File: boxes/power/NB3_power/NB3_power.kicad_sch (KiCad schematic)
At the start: 82 parts, among them J1 Barrel_Jack_PJ-036AH-SMT-TR, J2 Conn_01x02_Male, J3 Conn_01x02_Male, J4 Conn_01x02_Male, J5 Conn_01x04_Male, J6 Conn_01x02_Male, J7 Conn_01x02_Male, Q1 Q_PMOS_GDS, Q2 Q_NMOS_GDS, SW1 SW_SPDT, U1 NiMH_Charger_LTC4010, U2 Voltage_Regulator_AP64501

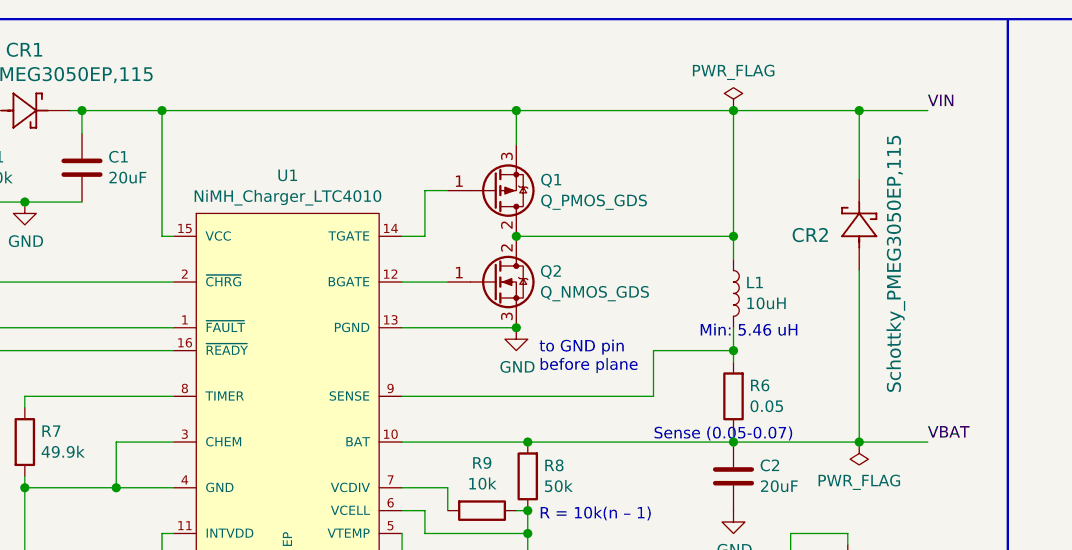
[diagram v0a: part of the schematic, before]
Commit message: More work on NB£_power PCB
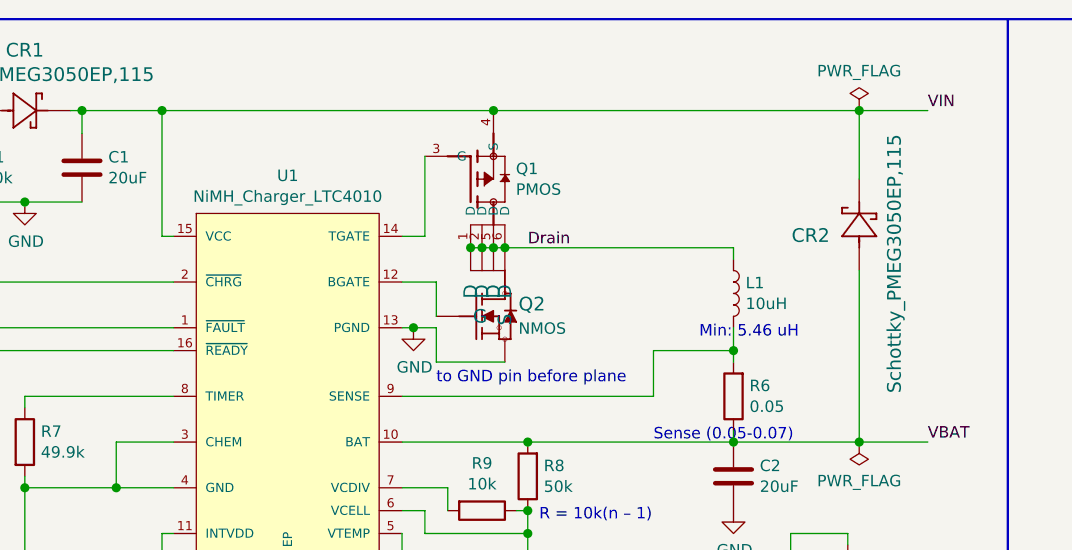
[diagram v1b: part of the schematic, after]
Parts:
- removed Q1: Q_PMOS_GDS, NB3_power:PMOS_SMD_FDC658AP, symbol Device:Q_PMOS_GDS
- removed Q2: Q_NMOS_GDS, NB3_power:NMOS_SMD_SI3410DV-T1-GE3, symbol Device:Q_NMOS_GDS
- added Q1: PMOS, NB3_power:PMOS_SMD_FDC658AP, symbol NB3_power:PMOS_SMD_FDC658AP
- added Q2: NMOS, NB3_power:NMOS_SMD_SI3410DV-T1-GE3, symbol NB3_power:NMOS_SMD_SI3410DV-T1-GE3
- J2, J3, J4, J6, J7: footprint Connector_PinHeader_2.54mm:PinHeader_1x02_P2.54mm_Vertical_SMD_Pin1Left -> Connector_PinHeader_2.54mm:PinHeader_1x02_P2.54mm_Vertical_SMD_Pin1Right
- J5: footprint Connector_PinHeader_2.54mm:PinHeader_1x04_P2.54mm_Vertical_SMD_Pin1Left -> Connector_PinHeader_2.54mm:PinHeader_1x04_P2.54mm_Vertical_SMD_Pin1Right
- L1: footprint Inductor_SMD:L_0805_2012Metric -> Inductor_SMD:L_Bourns_SRN6045TA
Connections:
- net GND: now also Q2.4 (S)
- net VIN: now also Q1.4 (S); no longer L1.1
- net at U1.12 (BGATE): now also Q2.3 (G)
- net at U1.14 (TGATE): now also Q1.3 (G)
- new net Drain: L1.1, Q1.1 (D), Q1.2 (D), Q1.5 (D), Q1.6 (D), Q2.1 (D), Q2.2 (D), Q2.5 (D), Q2.6 (D)
